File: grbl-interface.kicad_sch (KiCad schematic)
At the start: 12 parts, among them U6 USBLC6-2SC6, U7 ADUM4160, U8 ATmega16U2-A, U9 ATmega328P-A, Y1 Crystal_GND24

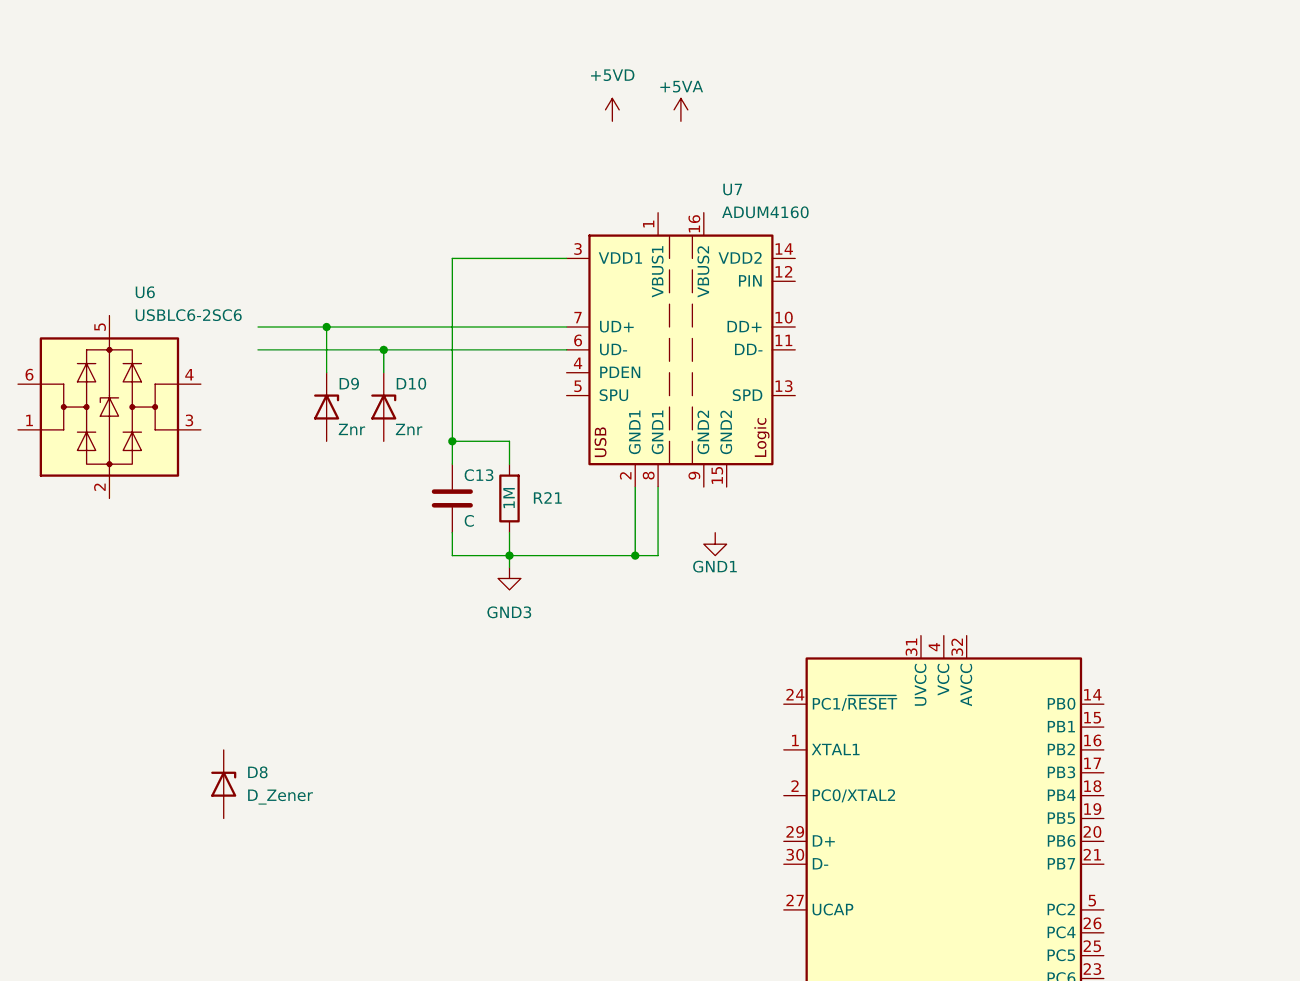
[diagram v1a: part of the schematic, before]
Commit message: wip
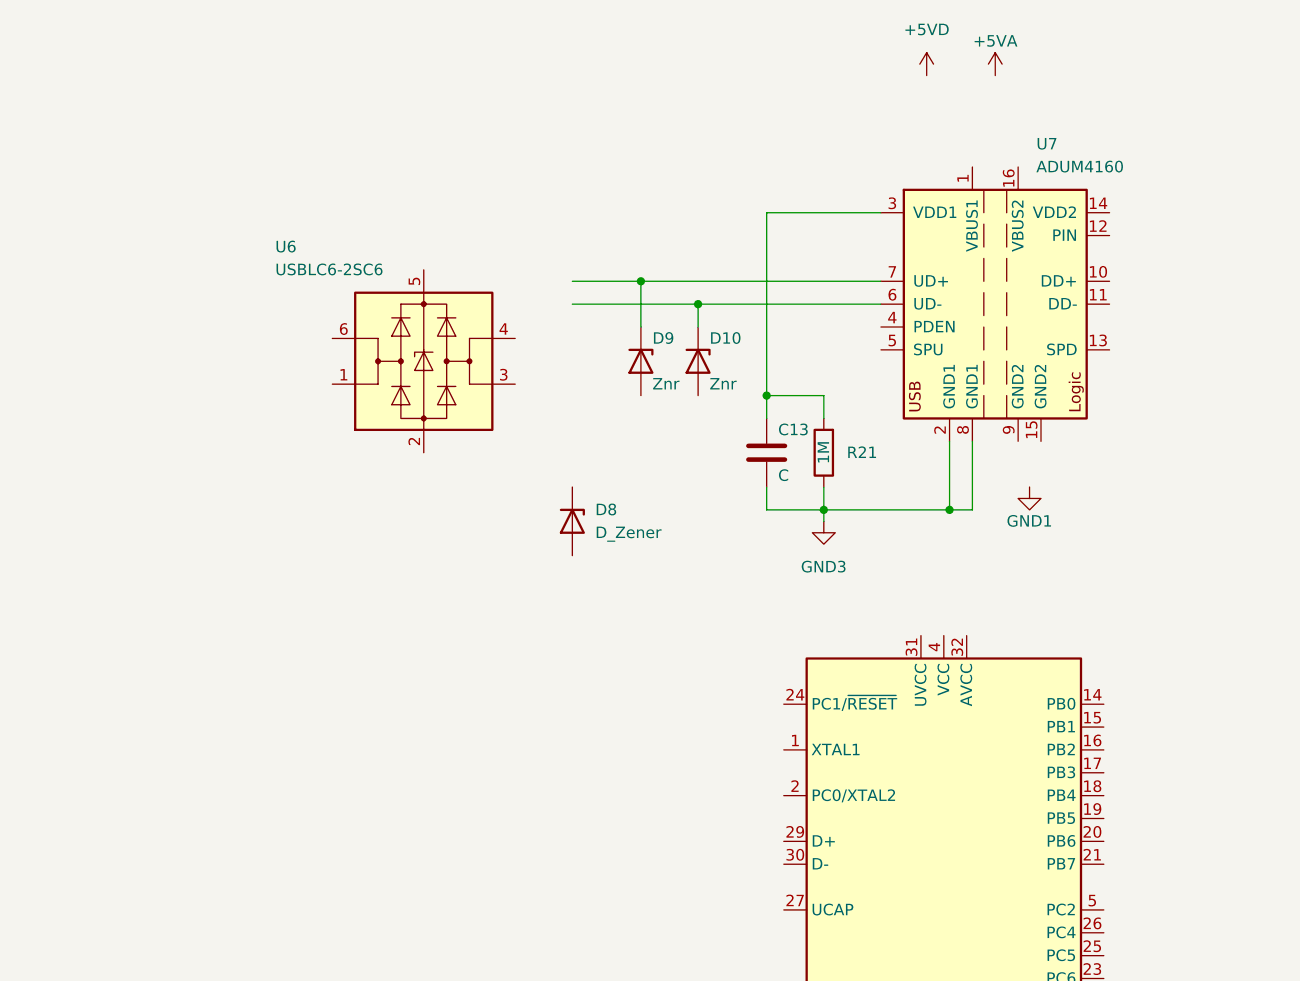
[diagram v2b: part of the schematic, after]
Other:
- moved on the sheet: C13, D10, D8, D9, R21, U6, U7
